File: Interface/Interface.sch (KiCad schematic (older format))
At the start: 3 parts, among them U1 SN74LVC1T45

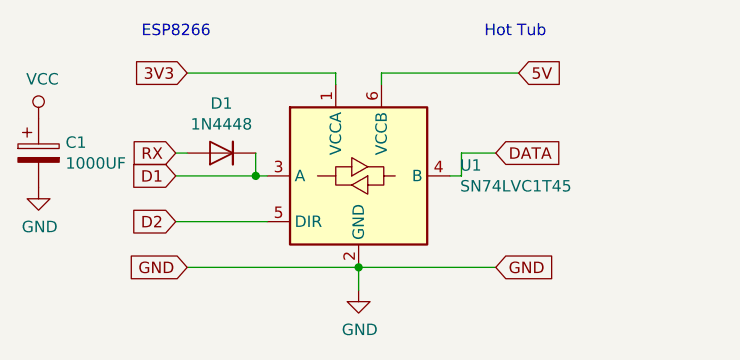
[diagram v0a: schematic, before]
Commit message: Updated schematic
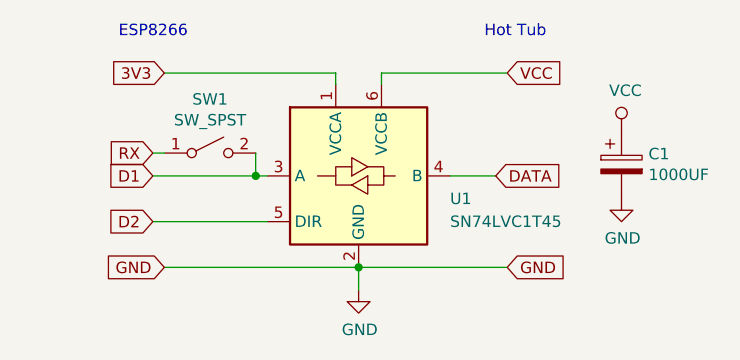
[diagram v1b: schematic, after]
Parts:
- removed D1: 1N4448, Diode_SMD:D_SOD-123, symbol Diode:1N4448W
- added SW1: SW_SPST, symbol Switch:SW_SPST
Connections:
- net 5V is gone; now on net VCC: U1.6 (VCCB)
- net D1: now also SW1.2 (B)
- net RX: now also SW1.1 (A)
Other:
- moved on the sheet: C1
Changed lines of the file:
@@
 L power:VCC #PWR?
 U 1 1 5D70837B
-P 3800 1700
-F 0 "#PWR?" H 3800 1550 50  0001 C CNN
-F 1 "VCC" H 3817 1873 50  0000 C CNN
-F 2 "" H 3800 1700 50  0001 C CNN
-F 3 "" H 3800 1700 50  0001 C CNN
-	1    3800 1700
+P 6350 1750
+F 0 "#PWR?" H 6350 1600 50  0001 C CNN
+F 1 "VCC" H 6367 1923 50  0000 C CNN
+F 2 "" H 6350 1750 50  0001 C CNN
+F 3 "" H 6350 1750 50  0001 C CNN
+	1    6350 1750
 	1    0    0    -1
 $EndComp
@@
 U 1 1 5E9CDB6D
 P 5200 1950
-F 0 "U1" H 5644 1996 50  0000 L CNN
-F 1 "SN74LVC1T45" H 5644 1905 50  0000 L CNN
+F 0 "U1" H 5600 1850 50  0000 L CNN
+F 1 "SN74LVC1T45" H 5600 1750 50  0000 L CNN
 F 2 "Package_TO_SOT_SMD:SOT-363_SC-70-6" H 5200 1500 50  0001 C CNN
 F 3 "http://www.ti.com/lit/ds/symlink/sn74lvc1t45.pdf" H 4300 1300 50  0001 C CNN
@@
 $EndComp
 Wire Wire Line
-	4400 2150 4800 2150
-Wire Wire Line
 	5300 1550 5300 1500
 Wire Wire Line
 	5100 1550 5100 1500
-Text GLabel 4400 1850 0    50   Input ~ 0
+Text GLabel 4300 1850 0    50   Input ~ 0
 RX
-Text GLabel 4400 1950 0    50   Input ~ 0
+Text GLabel 4300 1950 0    50   Input ~ 0
 D1
-Text GLabel 5800 1850 2    50   Input ~ 0
+Text GLabel 5800 1950 2    50   Input ~ 0
 DATA
-Text GLabel 5800 2350 2    50   Input ~ 0
+Text GLabel 5850 2350 2    50   Input ~ 0
 GND
-Text GLabel 4450 1500 0    50   Input ~ 0
+Text GLabel 4350 1500 0    50   Input ~ 0
 3V3
-Text GLabel 4400 2150 0    50   Input ~ 0
+Text GLabel 4300 2150 0    50   Input ~ 0
 D2
 Wire Wire Line
-	5100 1500 4450 1500
-Wire Wire Line
-	5200 2350 5800 2350
-Wire Wire Line
-	5600 1950 5650 1950
-Wire Wire Line
-	5650 1950 5650 1850
-Wire Wire Line
-	5650 1850 5800 1850
+	5200 2350 5850 2350
 $Comp
 L Device:CP C1
 U 1 1 5D708E3A
-P 3800 1850
-F 0 "C1" H 3918 1896 50  0000 L CNN
-F 1 "1000UF" H 3918 1805 50  0000 L CNN
-F 2 "" H 3838 1700 50  0001 C CNN
-F 3 "~" H 3800 1850 50  0001 C CNN
-	1    3800 1850
+P 6350 1900
+F 0 "C1" H 6468 1946 50  0000 L CNN
+F 1 "1000UF" H 6468 1855 50  0000 L CNN
+F 2 "" H 6388 1750 50  0001 C CNN
+F 3 "~" H 6350 1900 50  0001 C CNN
+	1    6350 1900
 	1    0    0    -1
 $EndComp
@@
 L power:GND #PWR?
 U 1 1 5D708717
-P 3800 2000
-F 0 "#PWR?" H 3800 1750 50  0001 C CNN
-F 1 "GND" H 3805 1827 50  0000 C CNN
-F 2 "" H 3800 2000 50  0001 C CNN
-F 3 "" H 3800 2000 50  0001 C CNN
-	1    3800 2000
+P 6350 2050
+F 0 "#PWR?" H 6350 1800 50  0001 C CNN
+F 1 "GND" H 6355 1877 50  0000 C CNN
+F 2 "" H 6350 2050 50  0001 C CNN
+F 3 "" H 6350 2050 50  0001 C CNN
+	1    6350 2050
 	1    0    0    -1
 $EndComp
@@
 	5200 2450 5200 2350
 Connection ~ 5200 2350
-$Comp
-L Diode:1N4448W D1
-U 1 1 5EA5CF14
-P 4600 1850
-F 0 "D1" H 4600 1633 50  0000 C CNN
-F 1 "1N4448" H 4600 1724 50  0000 C CNN
-F 2 "Diode_SMD:D_SOD-123" H 4600 1675 50  0001 C CNN
-F 3 "https://www.vishay.com/docs/85722/1n4448w.pdf" H 4600 1850 50  0001 C CNN
-	1    4600 1850
-	-1   0    0    1
-$EndComp
 Wire Wire Line
 	4750 1850 4750 1950
@@
 	4750 1950 4800 1950
 Wire Wire Line
-	4400 1950 4750 1950
-Connection ~ 4750 1950
+	4350 1850 4300 1850
 Wire Wire Line
-	4450 1850 4400 1850
-Wire Wire Line
-	5300 1500 5900 1500
-Text GLabel 5900 1500 2    50   Input ~ 0
-5V
-Text GLabel 4450 2350 0    50   Input ~ 0
+	5300 1500 5850 1500
+Text GLabel 5850 1500 2    50   Input ~ 0
+VCC
+Text GLabel 4350 2350 0    50   Input ~ 0
 GND
-Wire Wire Line
-	4450 2350 5200 2350
-Text Notes 4250 1350 0    50   ~ 0
+Text Notes 4150 1350 0    50   ~ 0
 ESP8266
 Text Notes 5750 1350 0    50   ~ 0
 Hot Tub
+Wire Wire Line
+	5600 1950 5800 1950
+$Comp
+L Switch:SW_SPST SW1
+U 1 1 5EB89F8D
+P 4550 1850
+F 0 "SW1" H 4550 2085 50  0000 C CNN
+F 1 "SW_SPST" H 4550 1994 50  0000 C CNN
+F 2 "" H 4550 1850 50  0001 C CNN
+F 3 "~" H 4550 1850 50  0001 C CNN
+	1    4550 1850
+	1    0    0    -1
+$EndComp
+Wire Wire Line
+	4750 1950 4300 1950
+Connection ~ 4750 1950
+Wire Wire Line
+	4300 2150 4800 2150
+Wire Wire Line
+	4350 2350 5200 2350
+Wire Wire Line
+	4350 1500 5100 1500
 $EndSCHEMATC
